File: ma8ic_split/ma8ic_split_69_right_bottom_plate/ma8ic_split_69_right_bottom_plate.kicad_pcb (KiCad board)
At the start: 2 copper layers, 166.3 x 125.7 mm, 9 parts

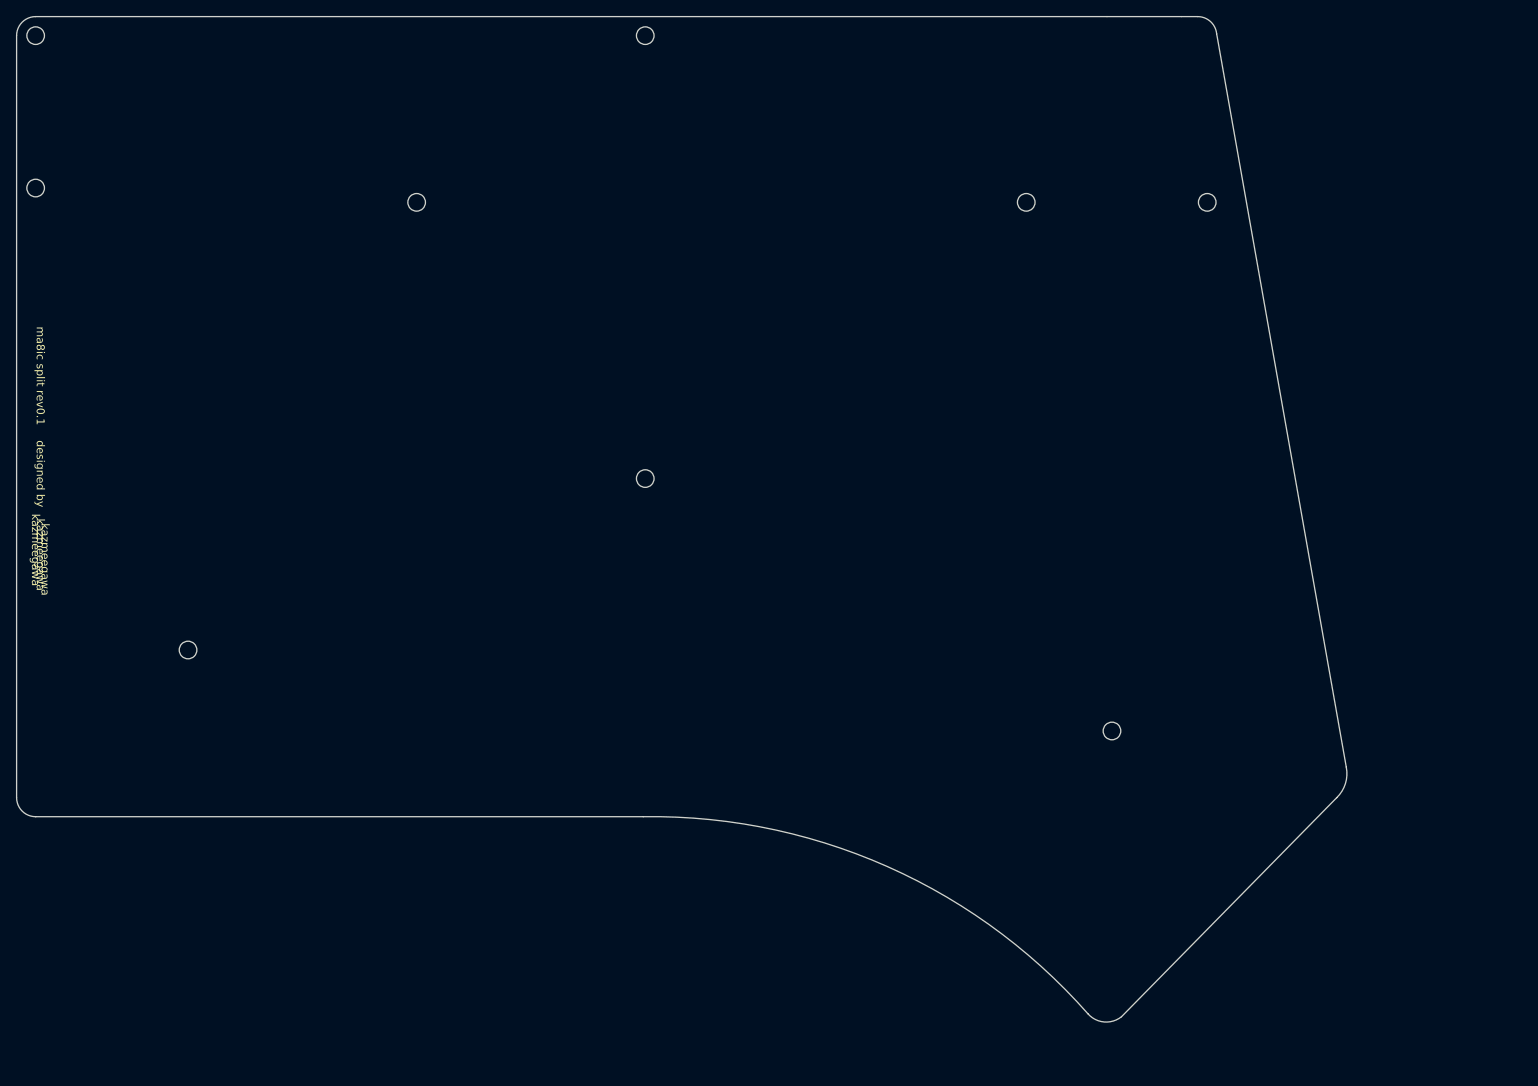
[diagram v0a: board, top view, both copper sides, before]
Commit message: update
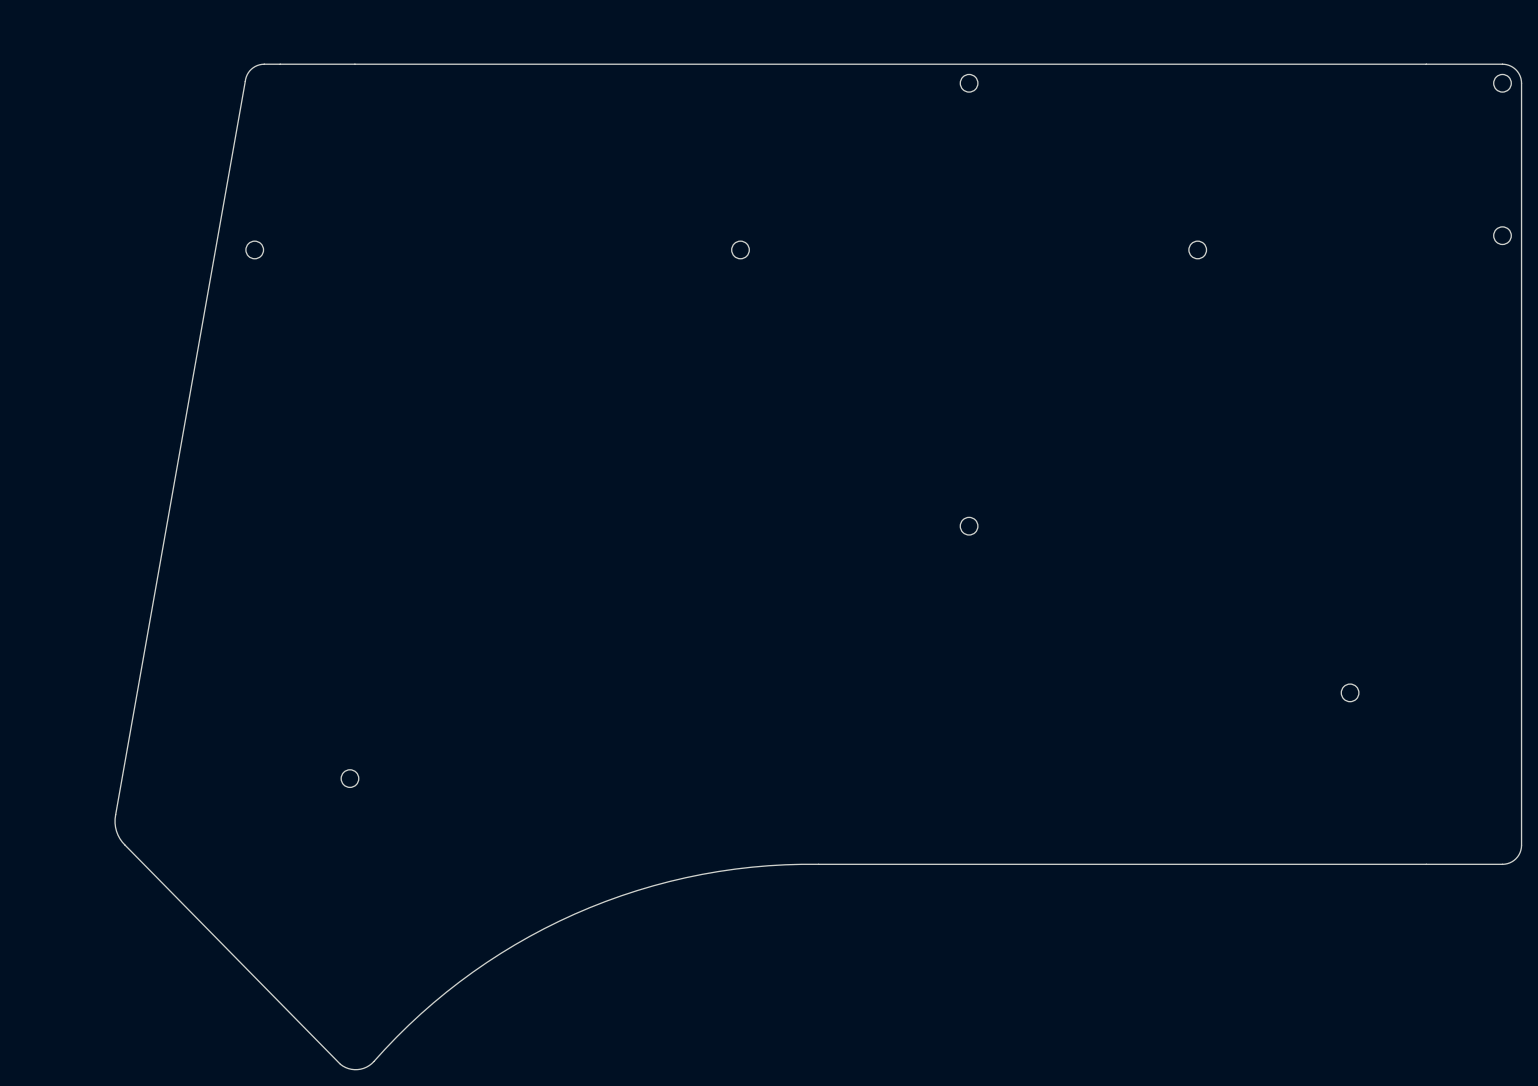
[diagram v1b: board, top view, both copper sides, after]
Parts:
- ? (x5), REF** (x4): moved to B.Cu
- moved ? 183.5 mm to (233.4, 38.1), turned to 180 degrees
- moved ? 183.5 mm to (233.4, 57.1), turned to 180 degrees
- moved REF** 145.4 mm to (214.3, 114.3), turned to 180 degrees
- moved ? 119.2 mm to (77.4, 58.9), turned to 180 degrees
- moved REF** 97.8 mm to (195.3, 58.9), turned to 180 degrees
- moved REF** 95.4 mm to (89.3, 125.0), turned to 180 degrees
- moved ? 40.9 mm to (166.7, 38.1), turned to 180 degrees
- moved ? 40.9 mm to (166.7, 93.5), turned to 180 degrees
- moved REF** 36.2 mm to (138.1, 58.9), turned to 180 degrees
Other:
- board size 166.3 x 125.7 mm -> 175.8 x 125.7 mm
- board text removed: "designed by"
- board text removed: "kazmeegawa"
- board text removed: "ma8ic split rev0.1"

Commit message: update
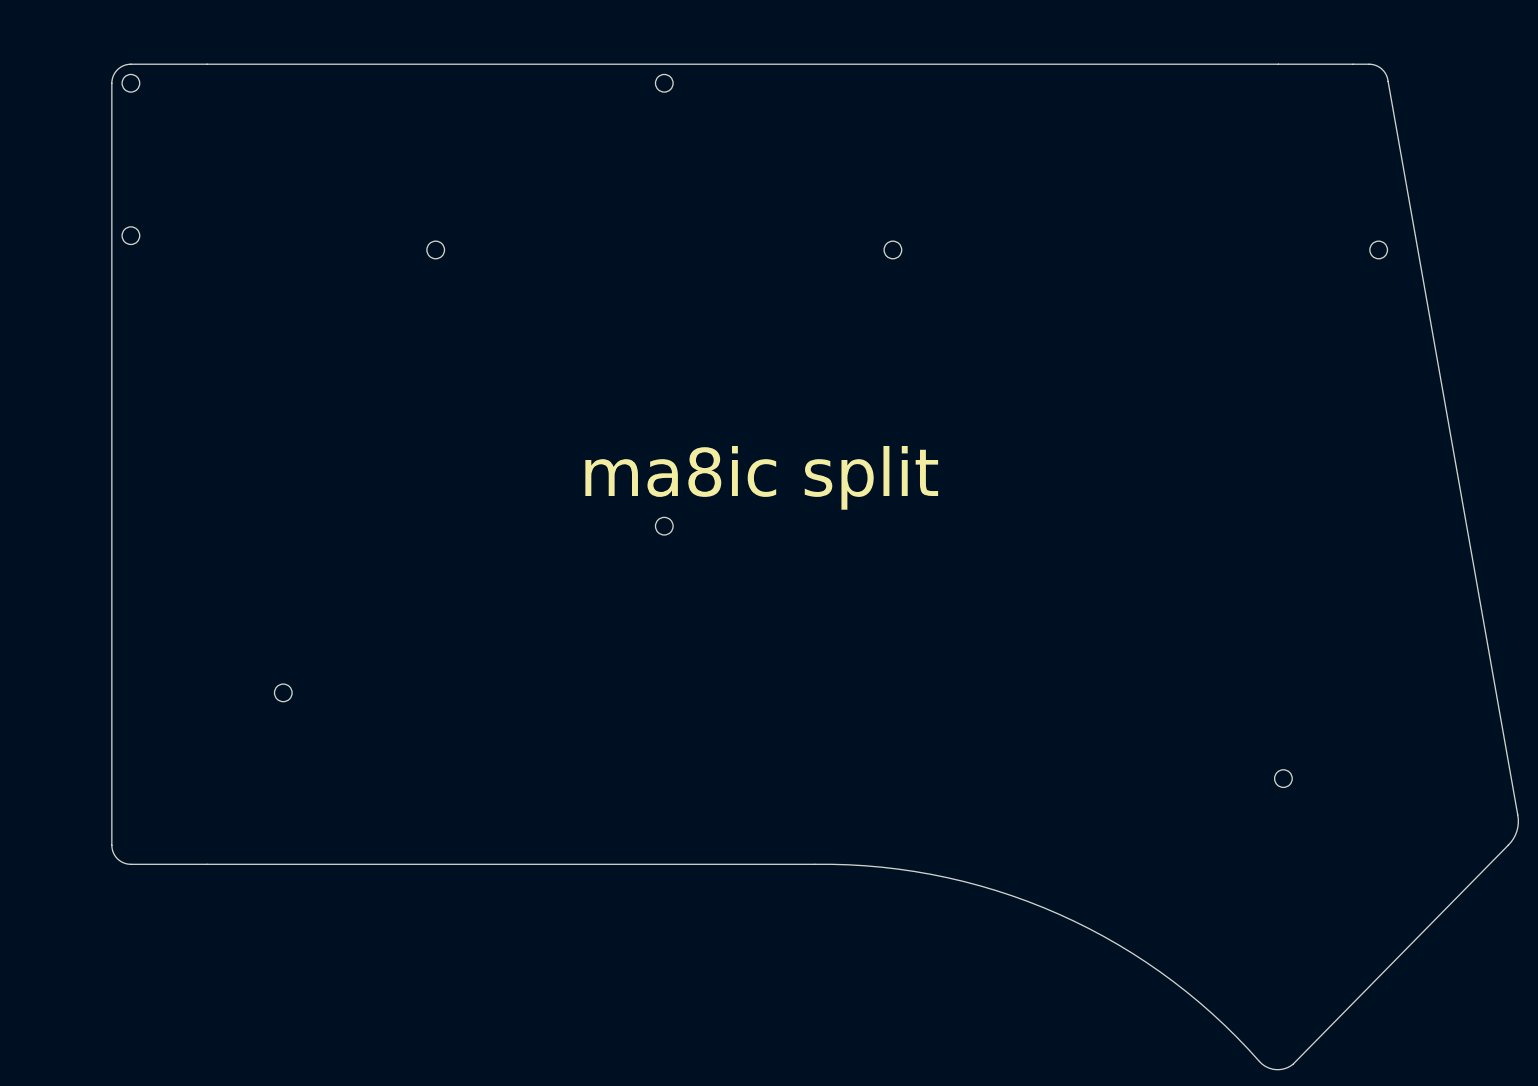
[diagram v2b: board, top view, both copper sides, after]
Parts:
- ? (x5), REF** (x4): moved to F.Cu
- moved ? 171.5 mm to (61.9, 38.1), turned to 0 degrees
- moved ? 171.5 mm to (61.9, 57.1), turned to 0 degrees
- moved ? 140.5 mm to (217.9, 58.9), turned to 0 degrees
- moved REF** 133.3 mm to (81.0, 114.3), turned to 0 degrees
- moved REF** 116.7 mm to (206.0, 125.0), turned to 0 degrees
- moved REF** 95.2 mm to (100.0, 58.9), turned to 0 degrees
- moved ? 38.1 mm to (128.6, 38.1), turned to 0 degrees
- moved ? 38.1 mm to (128.6, 93.5), turned to 0 degrees
- moved REF** 19.0 mm to (157.2, 58.9), turned to 0 degrees
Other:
- outline, holes or cut-outs redrawn
